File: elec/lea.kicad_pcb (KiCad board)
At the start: 2 copper layers, 76.2 x 76.2 mm, 9 parts, among them J1 Servomoteur, J2 Screw_Terminal_01x02, J3 Jack, SW1 SW_SPDT

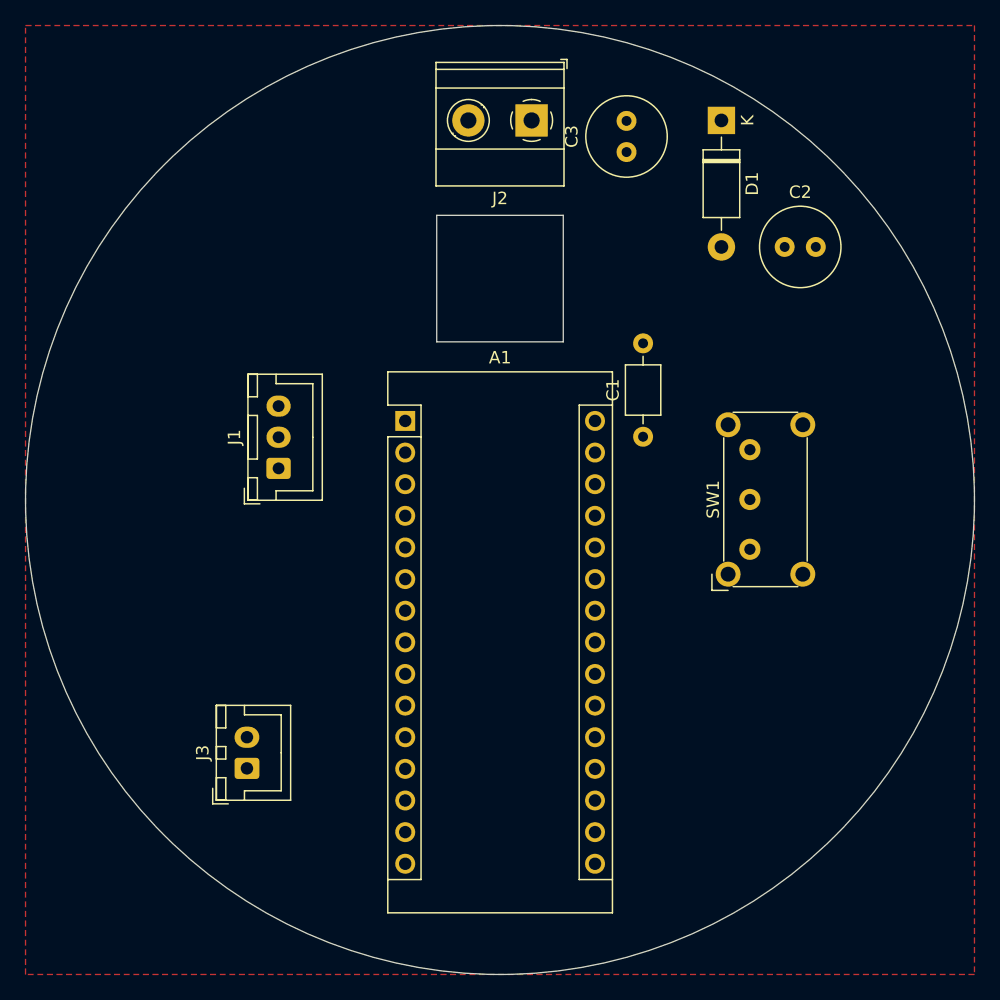
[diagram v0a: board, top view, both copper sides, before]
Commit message: commit avant changement de branche
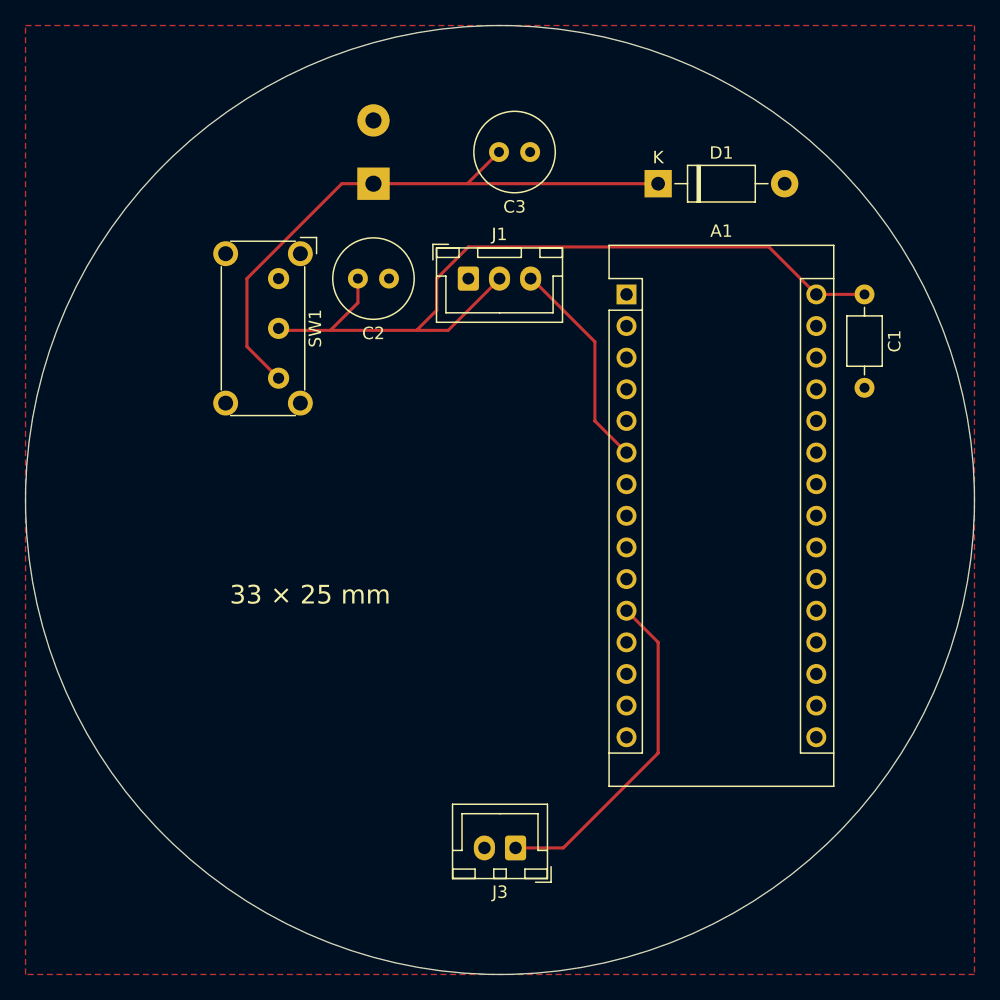
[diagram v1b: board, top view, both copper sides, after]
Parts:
- J2: moved to B.Cu
- moved SW1 43.6 mm to (101.6, 76.2), turned to -90 degrees
- moved C2 31.9 mm to (110.5, 76.2), turned to 180 degrees
- moved J3 22.5 mm to (120.6, 121.9), turned to 180 degrees
- moved J1 21.6 mm to (116.8, 76.2), turned to 0 degrees
- moved C1 21.1 mm to (148.7, 77.5), turned to -90 degrees
- moved A1 20.5 mm to (129.5, 77.5)
- moved J2 13.7 mm to (109.2, 68.6), turned to 90 degrees
- moved C3 7.74 mm to (121.8, 66.0), turned to 180 degrees
- moved D1 7.18 mm to (132.1, 68.6), turned to 0 degrees
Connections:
- J3 pad 1: GND -> /JCK
- J3 pad 2: /JCK -> GND
- SW1 pad 1: +9V -> unconnected-(SW1-Pad1)
- SW1 pad 3: unconnected-(SW1-Pad3) -> +9V
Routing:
- net /VIN: track 0.00 -> 66.4 mm
- net +9V: track 0.00 -> 48.8 mm
- net /JCK: track 0.00 -> 27.1 mm
- net /PWM: track 0.00 -> 17.2 mm
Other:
- outline, holes or cut-outs redrawn
- board text added: "33 × 25 mm"
